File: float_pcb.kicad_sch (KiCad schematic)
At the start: 34 parts, among them J1 BR Switch, J2 5V, J3 USB_C, J4 Servo, SW2 SW_Push, SW3 ENABLE, U1 TPSM863252RDXR, U2 TPSM863252RDXR, U3 ESP32-S3-MINI-1U

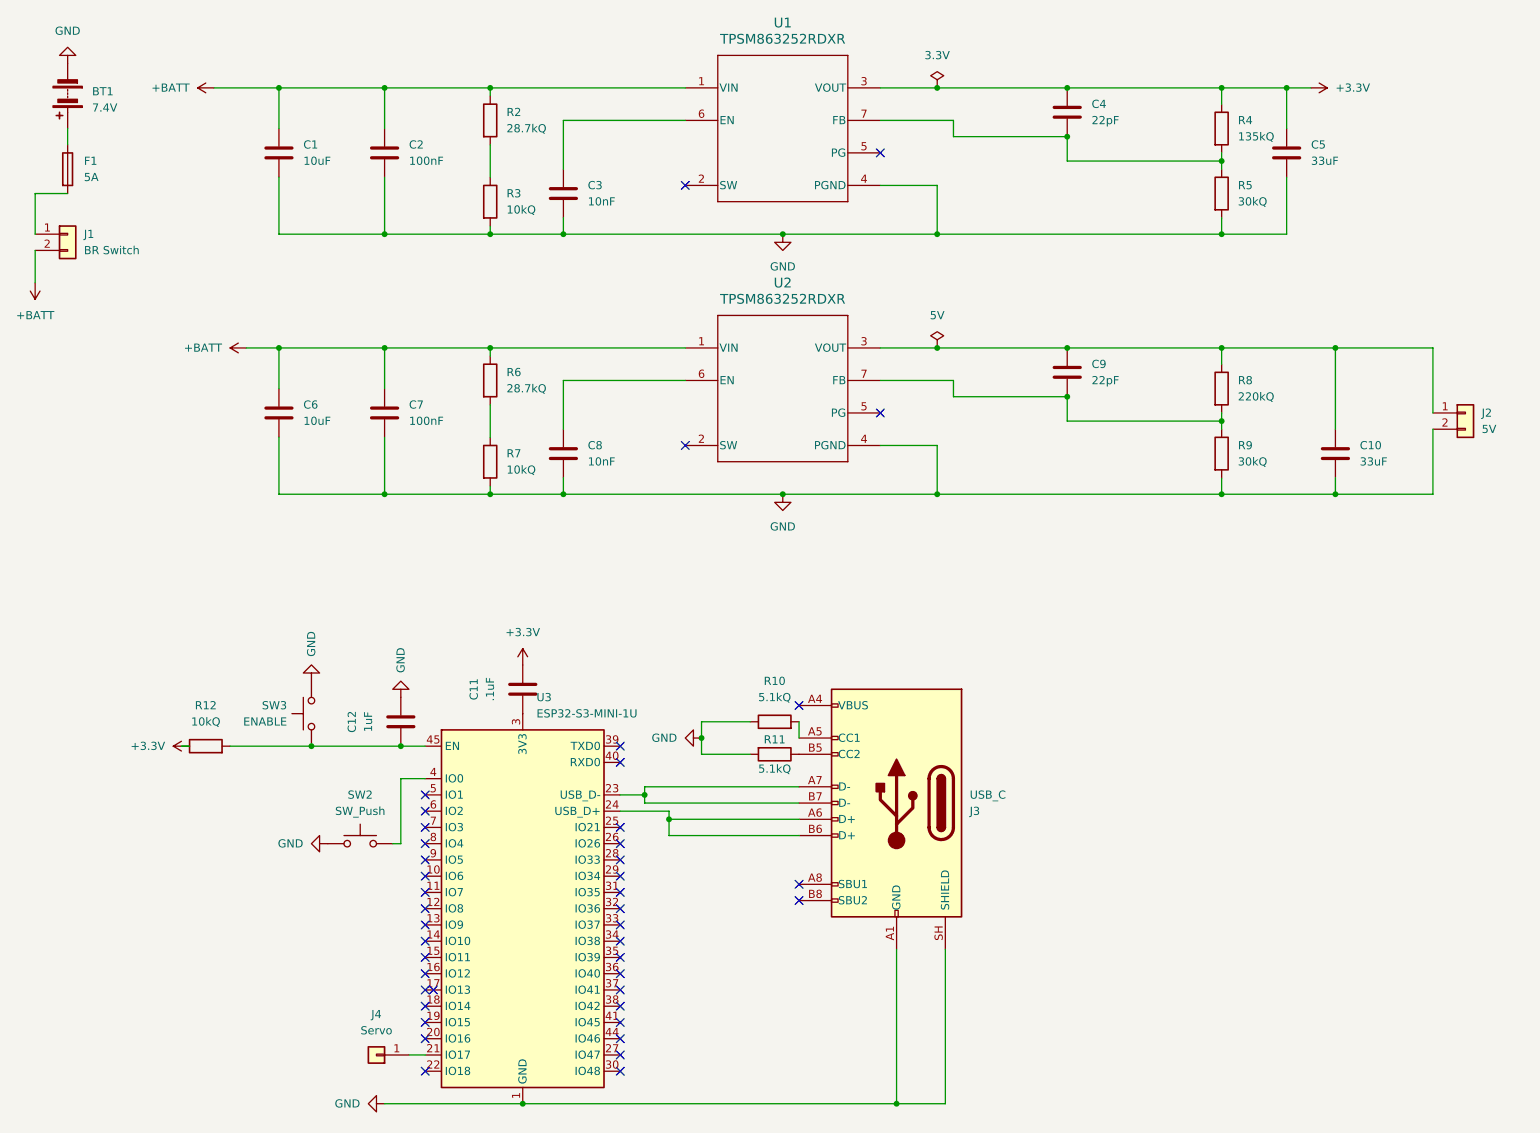
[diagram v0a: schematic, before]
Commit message: Add some things
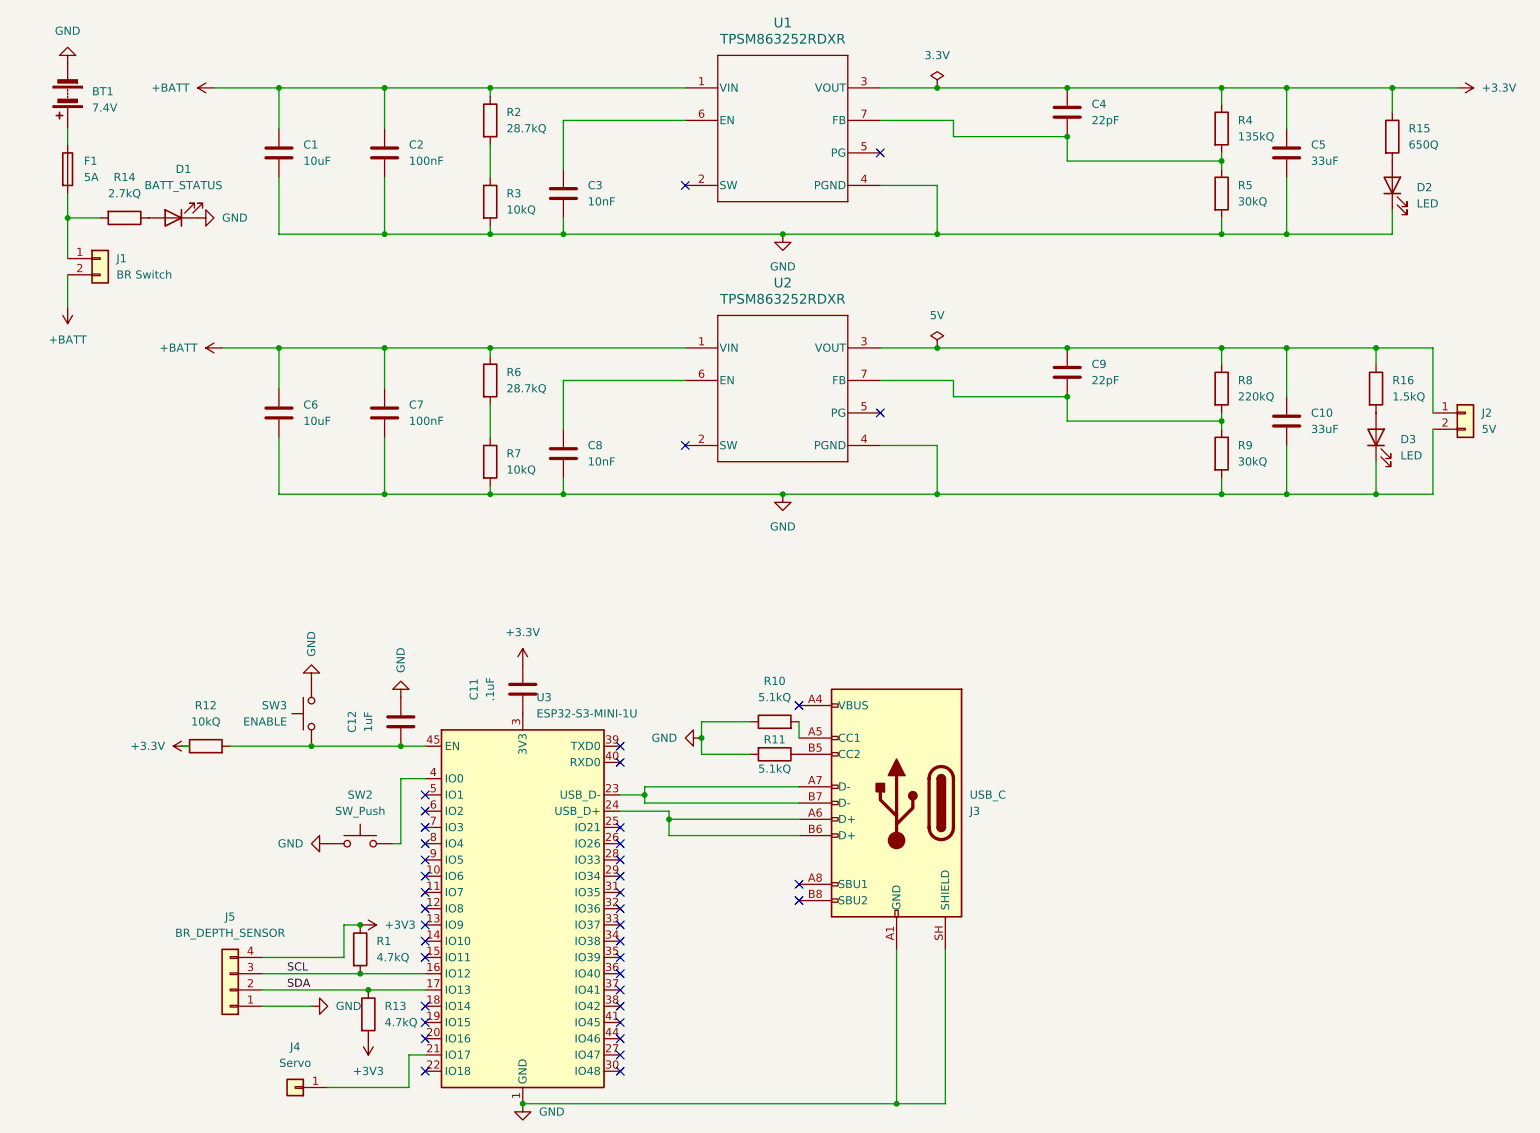
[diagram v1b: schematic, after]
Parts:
- added D1: BATT_STATUS, symbol Device:LED
- added D2, D3: LED, symbol Device:LED
- added J5: BR_DEPTH_SENSOR, Connector_JST:JST_GH_BM03B-GHS-TBT_1x03-1MP_P1.25mm_Vertical, symbol Connector_Generic:Conn_01x04
- added R1, R13: 4.7kQ, symbol Device:R
- added R14: 2.7kQ, symbol Device:R
- added R15: 650Q, symbol Device:R
- added R16: 1.5kQ, symbol Device:R
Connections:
- net +3.3V: now also R15.1
- net GND: now also D1.1 (K), D2.1 (K), D3.1 (K), J5.1 (Pin_1)
- net at C10.1, C9.1, J2.1 (Pin_1)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: now also R16.1
- net at F1.2, J1.1 (Pin_1): now also R14.2
- net SCL: now reaches U3.16 (IO12)
- net SCL: now also J5.3 (Pin_3), R1.2
- net SDA: now reaches U3.17 (IO13)
- net SDA: now also J5.2 (Pin_2), R13.1
- new net: D3.2 (A), R16.2
- new net: D2.2 (A), R15.2
- new net: D1.2 (A), R14.1
- new net +3V3: J5.4 (Pin_4), R1.1, R13.2
- no-connect marks 43 -> 40
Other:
- moved on the sheet: C10, J1, J4
